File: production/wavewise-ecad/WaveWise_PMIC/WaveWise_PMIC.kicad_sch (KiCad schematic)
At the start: 0 parts

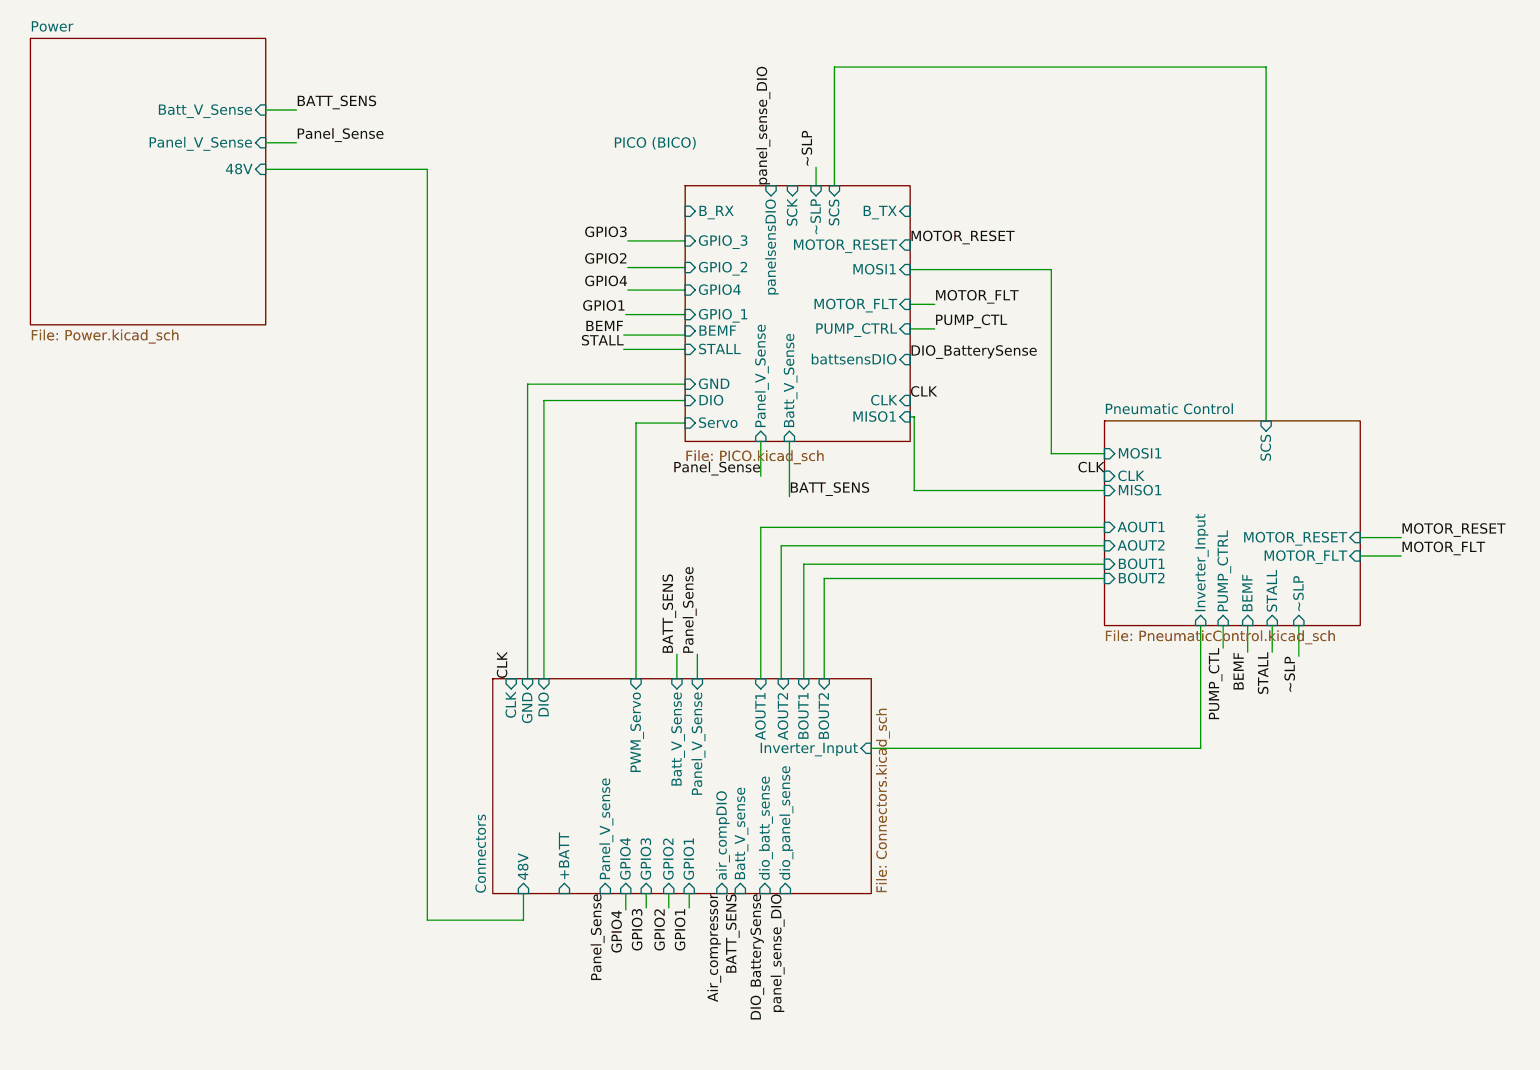
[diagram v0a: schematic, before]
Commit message: Prelim board layout
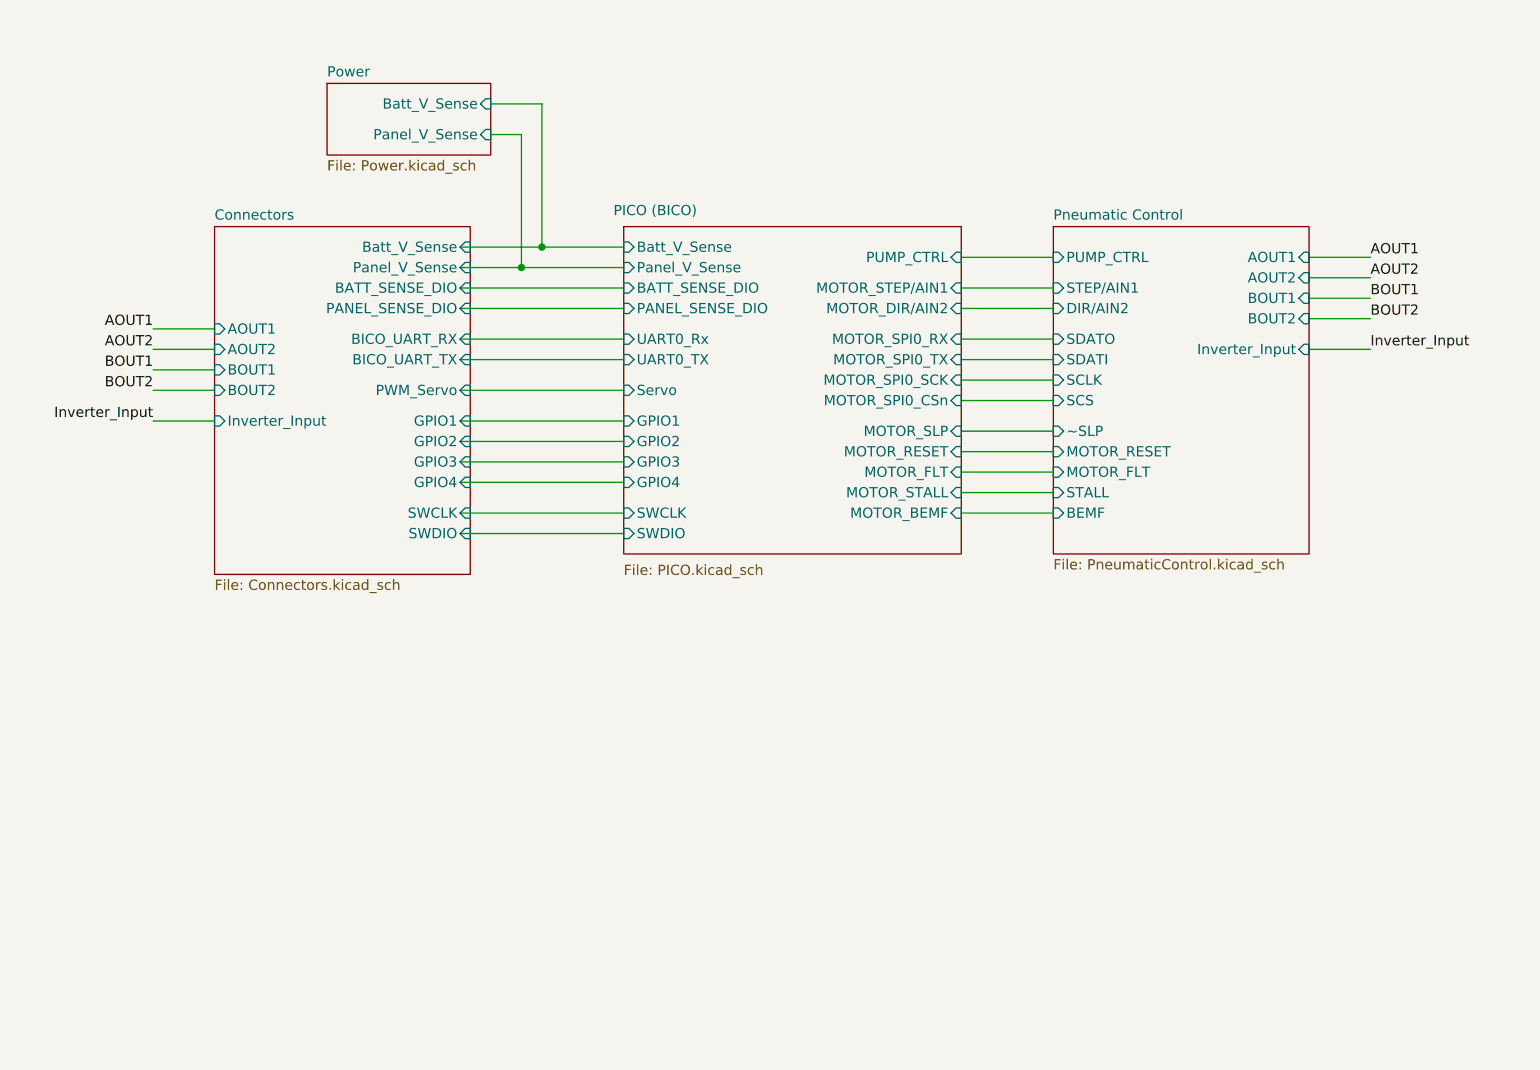
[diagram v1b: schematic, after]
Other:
- sheet Connectors ports: added BATT_SENSE_DIO, BICO_UART_RX, BICO_UART_TX, PANEL_SENSE_DIO, SWCLK, SWDIO; removed +BATT, 48V, Batt_V_sense, CLK, DIO, GND, Panel_V_sense, air_compDIO, dio_batt_sense, dio_panel_sense
- sheet PICO (BICO) ports: added BATT_SENSE_DIO, GPIO1, GPIO2, GPIO3, MOTOR_BEMF, MOTOR_DIR/AIN2, MOTOR_SLP, MOTOR_SPI0_CSn, MOTOR_SPI0_RX, MOTOR_SPI0_SCK, MOTOR_SPI0_TX, MOTOR_STALL, MOTOR_STEP/AIN1, PANEL_SENSE_DIO, SWCLK, SWDIO, UART0_Rx, UART0_TX; removed BEMF, B_RX, B_TX, CLK, DIO, GND, GPIO_1, GPIO_2, GPIO_3, MISO1, MOSI1, SCK, SCS, STALL, battsensDIO, panelsensDIO, ~SLP
- sheet Pneumatic Control ports: added DIR/AIN2, SCLK, SDATI, SDATO, STEP/AIN1; removed CLK, MISO1, MOSI1
- sheet Power ports: added none; removed 48V
